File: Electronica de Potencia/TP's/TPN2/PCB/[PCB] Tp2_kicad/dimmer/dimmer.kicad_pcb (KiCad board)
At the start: 2 copper layers, 62.6 x 43 mm, 20 parts, among them J1 Conn_01x02, J2 Conn_01x02, Q1 2N2647, Q2 TIC106

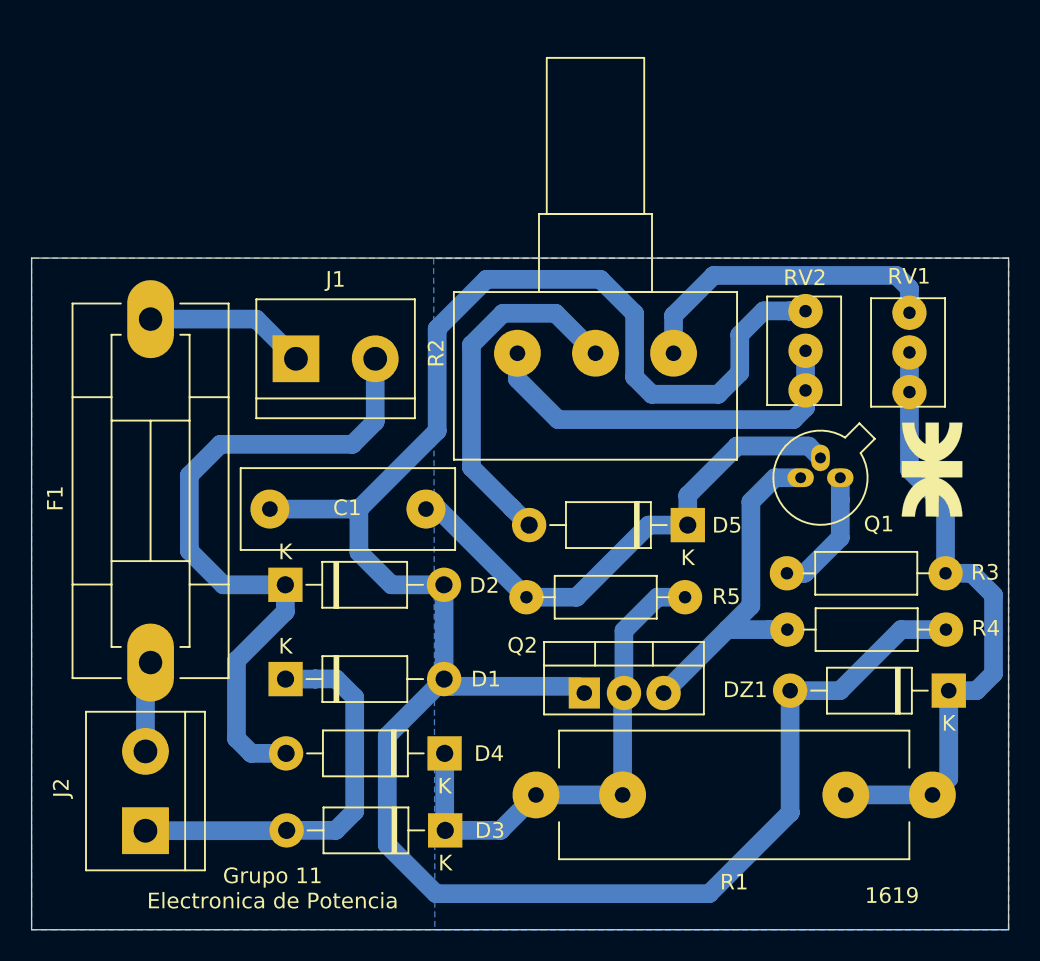
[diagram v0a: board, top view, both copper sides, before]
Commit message: Rediseño dimmer
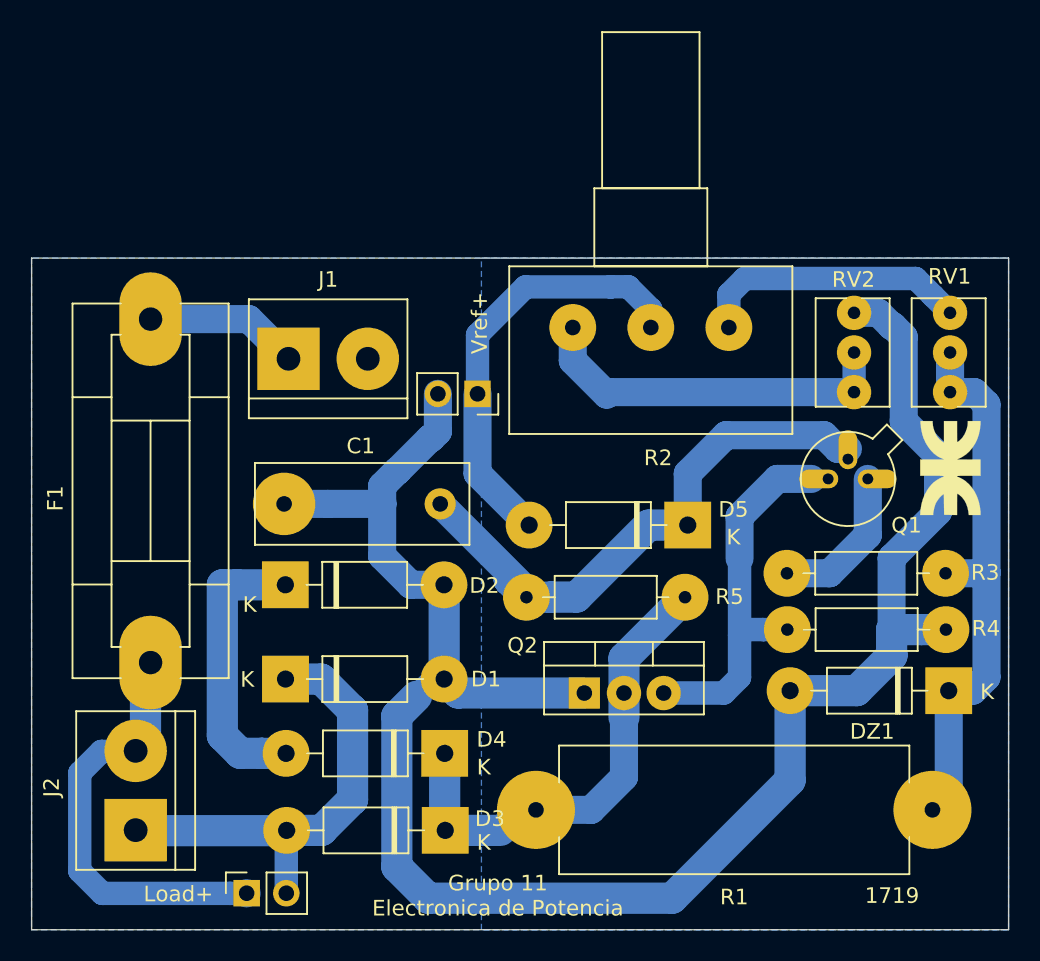
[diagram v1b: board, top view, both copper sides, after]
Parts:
- added Load+: TestPoint_2Pole, lib_fp:PinSocket_1x02_P2.54mm_Vertical, F.Cu at (133.4, 129.7)
- added Vref+: TestPoint_2Pole, lib_fp:PinSocket_1x02_P2.54mm_Vertical, F.Cu at (148.2, 97.8)
- J1: value Conn_01x02 -> Vin
- J2: value Conn_01x02 -> Vout
- moved R2 3.91 mm to (164.3, 93.5)
- moved RV2 3.11 mm to (172.3, 97.6)
- moved RV1 2.60 mm to (178.5, 97.6)
- moved Q1 1.76 mm to (173.2, 103.2)
- moved G1 1.18 mm to (178.5, 102.5)
- moved C1 0.97 mm to (145.8, 104.8)
- moved R1 0.96 mm to (151.9, 124.4)
- moved J2 0.63 mm to (126.3, 125.7)
- moved J1 0.48 mm to (136.1, 95.5)
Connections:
- net Net-(C1-Pad2) renamed /Vref-
- net Net-(D1-Pad1) renamed /Load-
- net Net-(D5-Pad2) renamed /Vref+
- net Net-(F1-Pad2) renamed /Load+
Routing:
- net GND: track 44.0 -> 18.3 mm
- net /Load+: track 6.18 -> 28.2 mm
- net /Vref-: track 138.6 -> 124.2 mm
- net /Vref+: track 22.9 -> 27.7 mm
- net Net-(C1-Pad1): track 33.1 -> 37.1 mm
- net Net-(DZ1-Pad1): track 39.8 -> 36.2 mm
- net Net-(R2-Pad1): track 20.5 -> 17.6 mm
- net /Load-: track 26.1 -> 29.0 mm
- net Net-(Q1-Pad2): track 22.3 -> 24.4 mm
- net Net-(D3-Pad1): track 32.6 -> 31.0 mm
- net Net-(Q1-Pad3): track 8.20 -> 9.79 mm
- net Net-(R2-Pad3): track 25.1 -> 23.7 mm
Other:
- net class Default: trace_width 1.2 -> 1.8
- board text added: "1719"
- board text removed: "1619"
